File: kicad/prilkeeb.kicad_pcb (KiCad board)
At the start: 2 copper layers, 196.9 x 158.6 mm, 73 parts, among them U2 Nice_Nano_V2

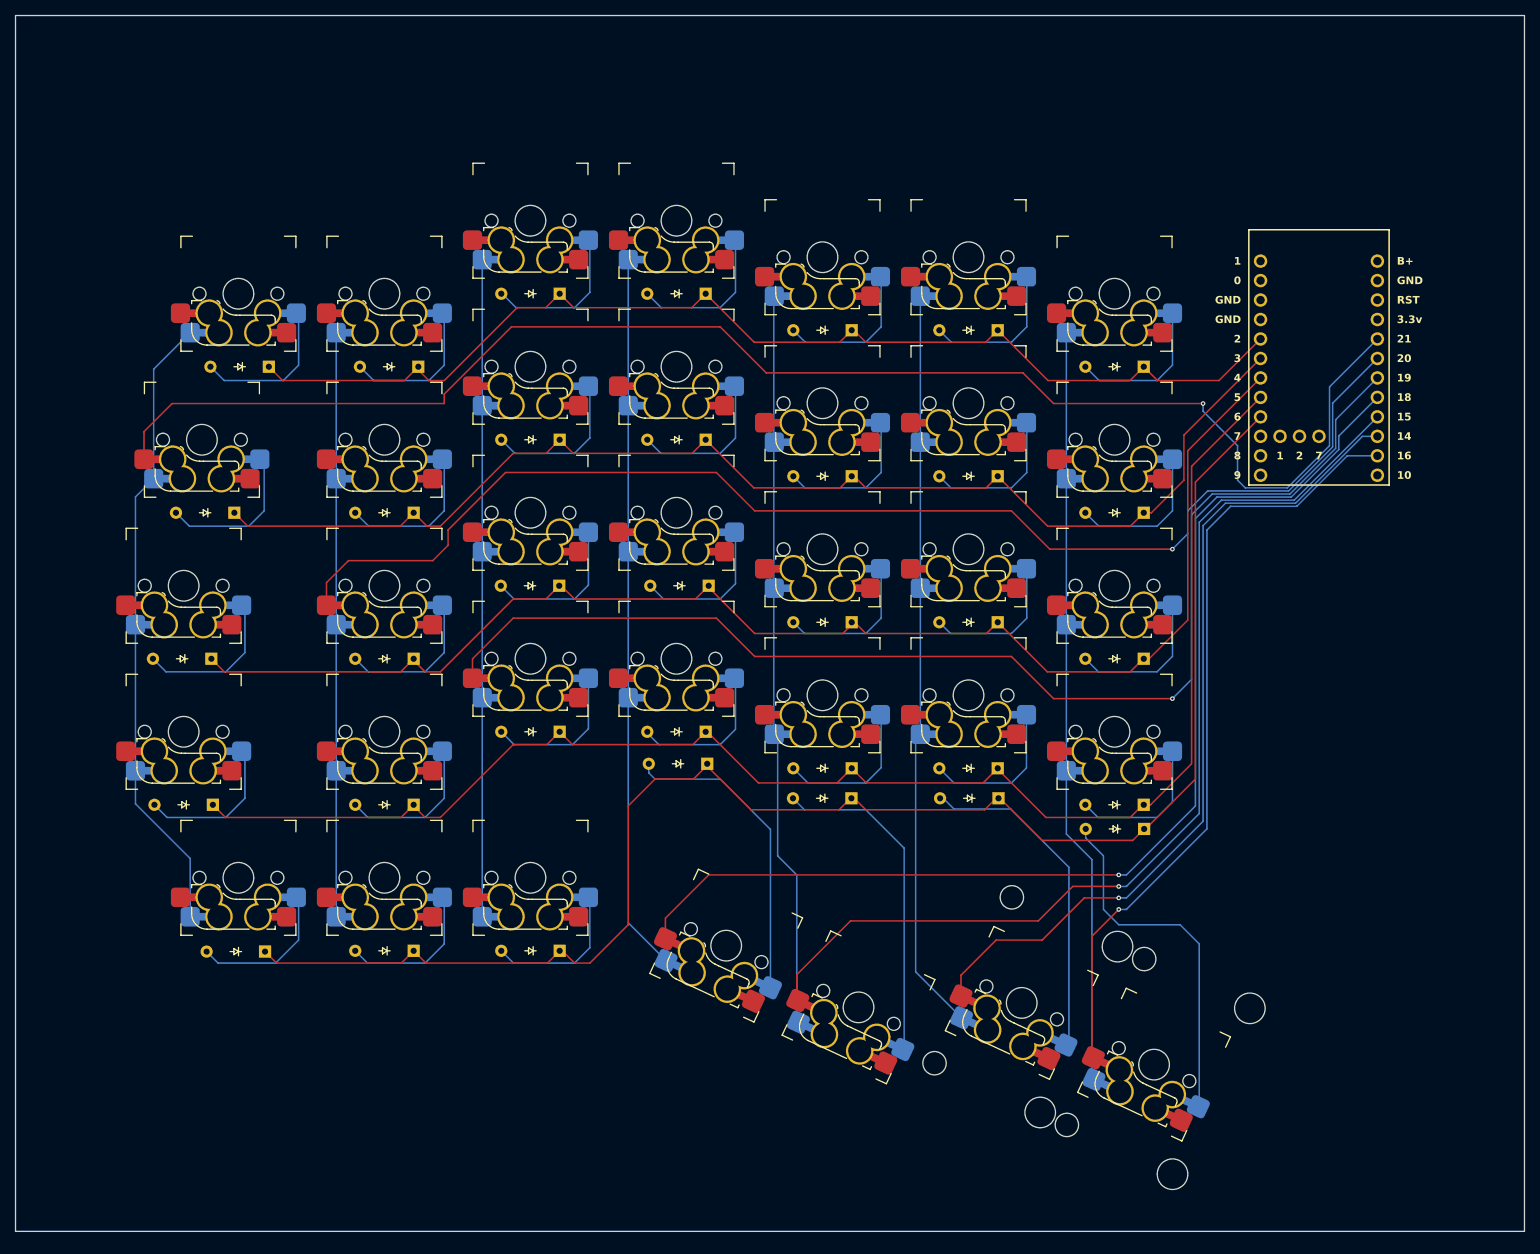
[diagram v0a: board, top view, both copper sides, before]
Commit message: Update layout
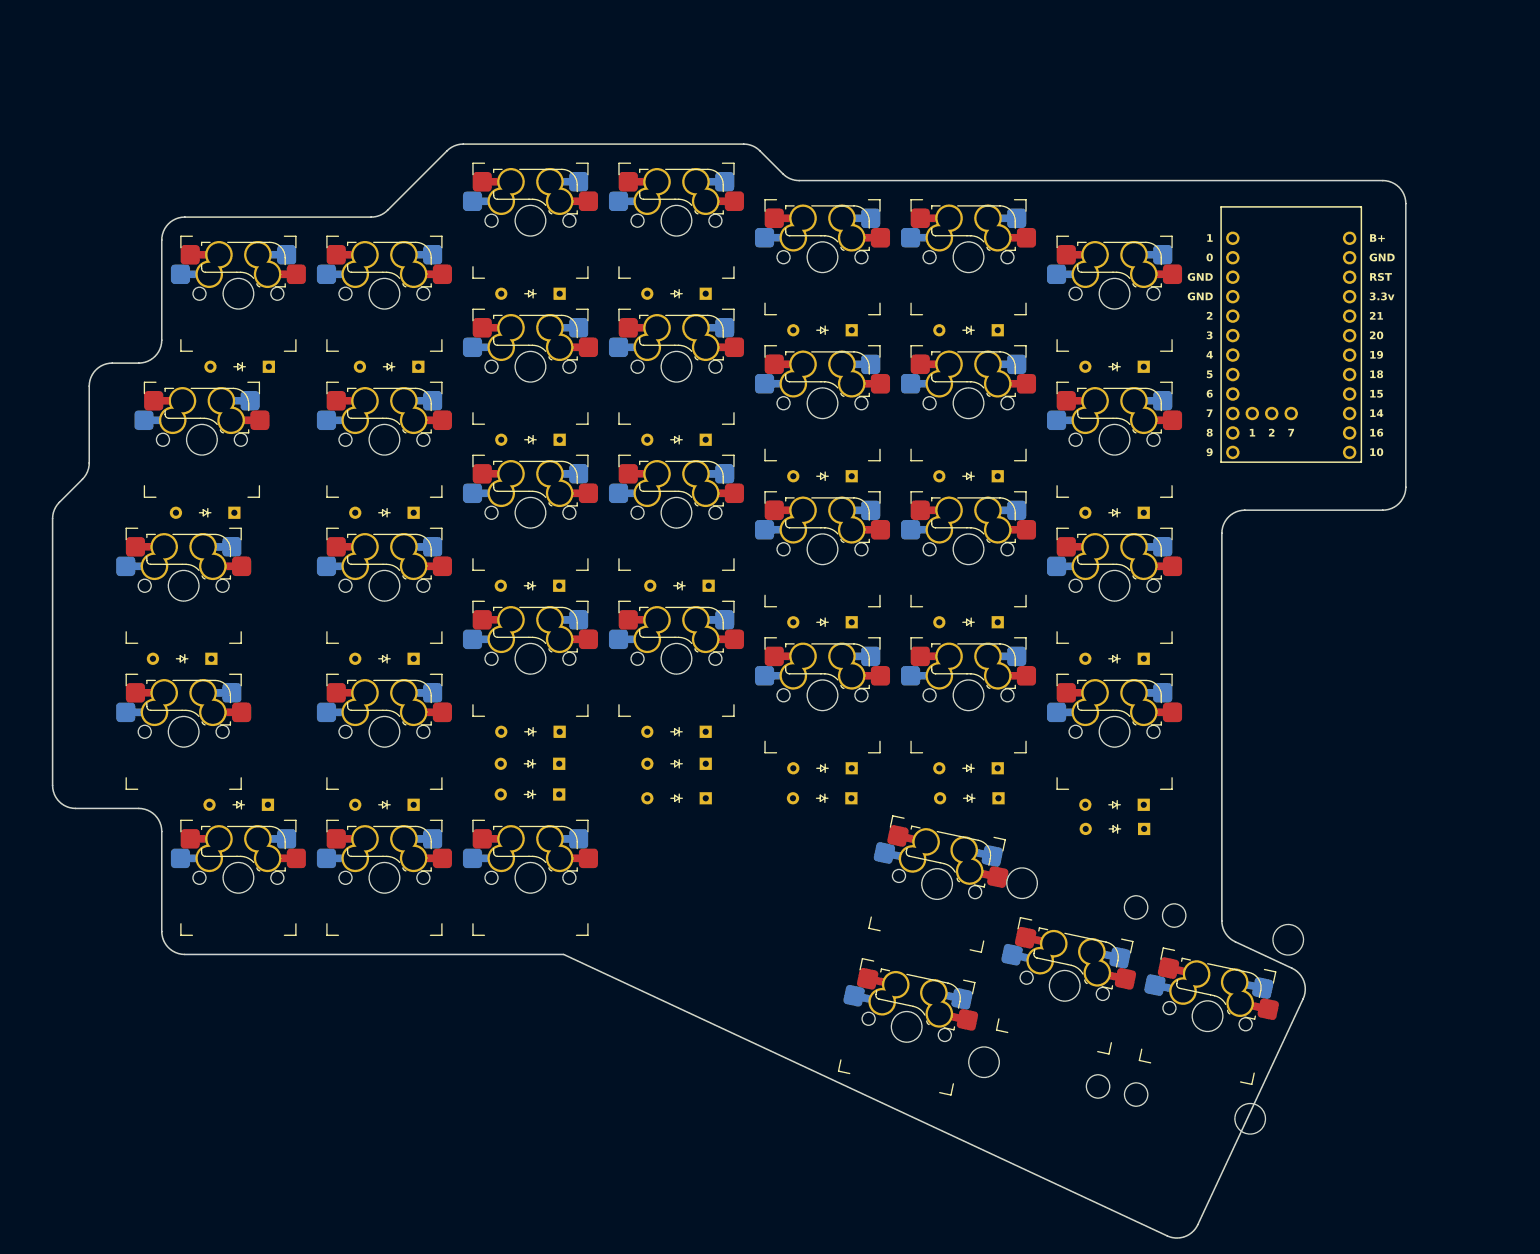
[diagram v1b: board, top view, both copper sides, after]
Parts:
- moved D29 43.5 mm to (99.0, 132.0)
- moved D30 30.9 mm to (99.0, 128.0)
- moved D31 27.6 mm to (118.1, 132.5)
- moved S35 25.8 mm to (144.3, 162.3), turned to -12 degrees
- moved S32 19.1 mm to (148.3, 143.7), turned to -12 degrees
- moved   9.41 mm to (183.6, 160.9), turned to 78 degrees
- moved S34 9.41 mm to (183.6, 160.9), turned to -12 degrees
- moved D22 7.18 mm to (61.0, 133.3)
- moved   6.04 mm to (164.9, 157.0), turned to -102 degrees
- moved S33 6.04 mm to (164.9, 157.0), turned to -12 degrees
- moved U2 4.69 mm to (194.5, 73.1)
- moved D32 0.19 mm to (118.1, 128.0)
- renumbered S35 to S32, S32 to S33, S33 to S34, S34 to S35
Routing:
- net Col_1: track 277.5 -> 0.00 mm, vias 1 -> 0
- net Col_3: track 245.0 -> 0.00 mm, vias 1 -> 0
- net Col_2: track 242.9 -> 0.00 mm, vias 1 -> 0
- net Col_4: track 240.2 -> 0.00 mm, vias 1 -> 0
- net Col_5: track 227.8 -> 0.00 mm, vias 1 -> 0
- net Col_6: track 205.6 -> 0.00 mm, vias 1 -> 0
- net Row_5: track 205.5 -> 0.00 mm
- net Col_7: track 200.9 -> 0.00 mm, vias 1 -> 0
- net Row_4: track 198.1 -> 0.00 mm
- net Row_3: track 181.4 -> 0.00 mm
- net Row_2: track 161.9 -> 0.00 mm
- net Row_1: track 149.1 -> 0.00 mm
- net Net-(D34-A): track 47.1 -> 0.00 mm
- net Net-(D33-A): track 43.9 -> 0.00 mm
- net Net-(D35-A): track 43.5 -> 0.00 mm
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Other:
- board size 196.9 x 158.6 mm -> 176.5 x 142.7 mm
